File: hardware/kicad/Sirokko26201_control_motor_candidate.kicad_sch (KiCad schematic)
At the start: 35 parts, among them J1 DEVKITC1_J1, J10 TC_K_EXHAUST_T+_T-, J11 TC_K_AIR_T+_T-, J12 ROOM_DS18B20_HARNESS, J13 24V_INPUT_PHOENIX_1756993_WIP, J27 GLOW_OUTPUT_PHOENIX_1756993, J28 CLUTCH_OUTPUT_PHOENIX_1756993, J3 DEVKITC1_J3, K1 DG85BM-5021-76-1024 + DZ85AB-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, K2 DG85BM-5021-76-1024 + DZ85AB-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, Q20 BC847B,215, U10 MAX31856MUD+, U20 SN74LVC1G97DBVR, U9 MAX31856MUD+

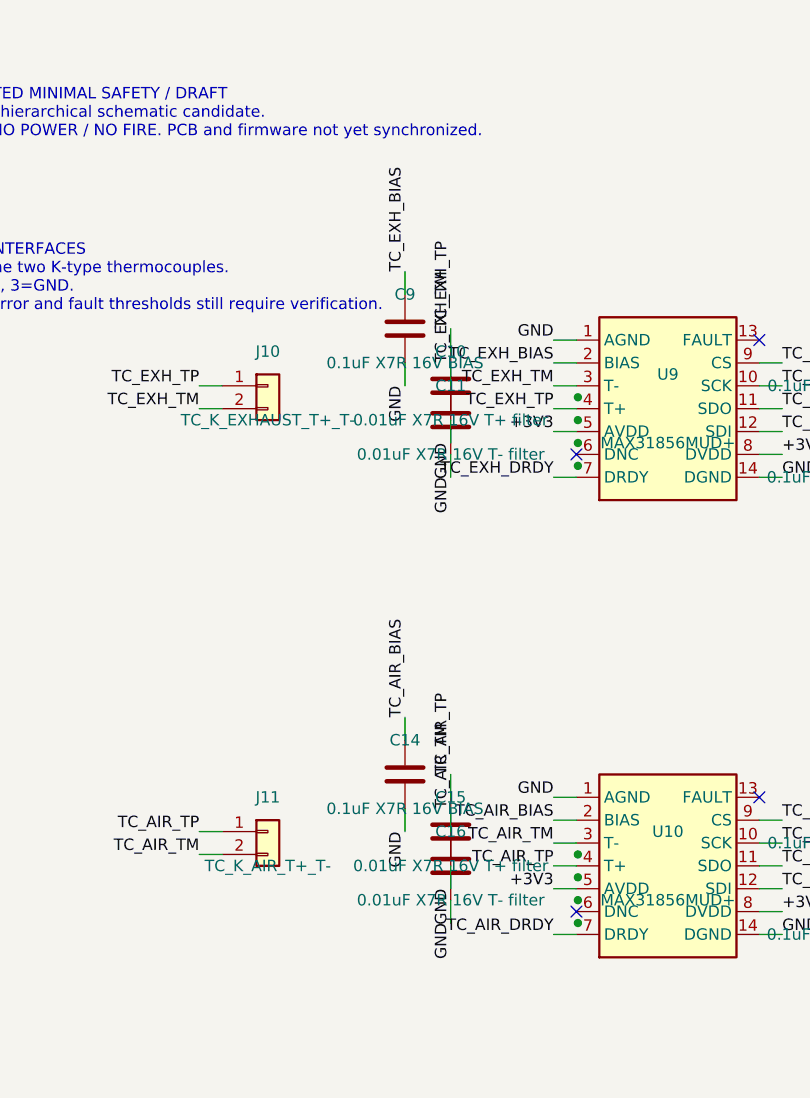
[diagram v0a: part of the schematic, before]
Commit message: Publish thermocouple correction draft package
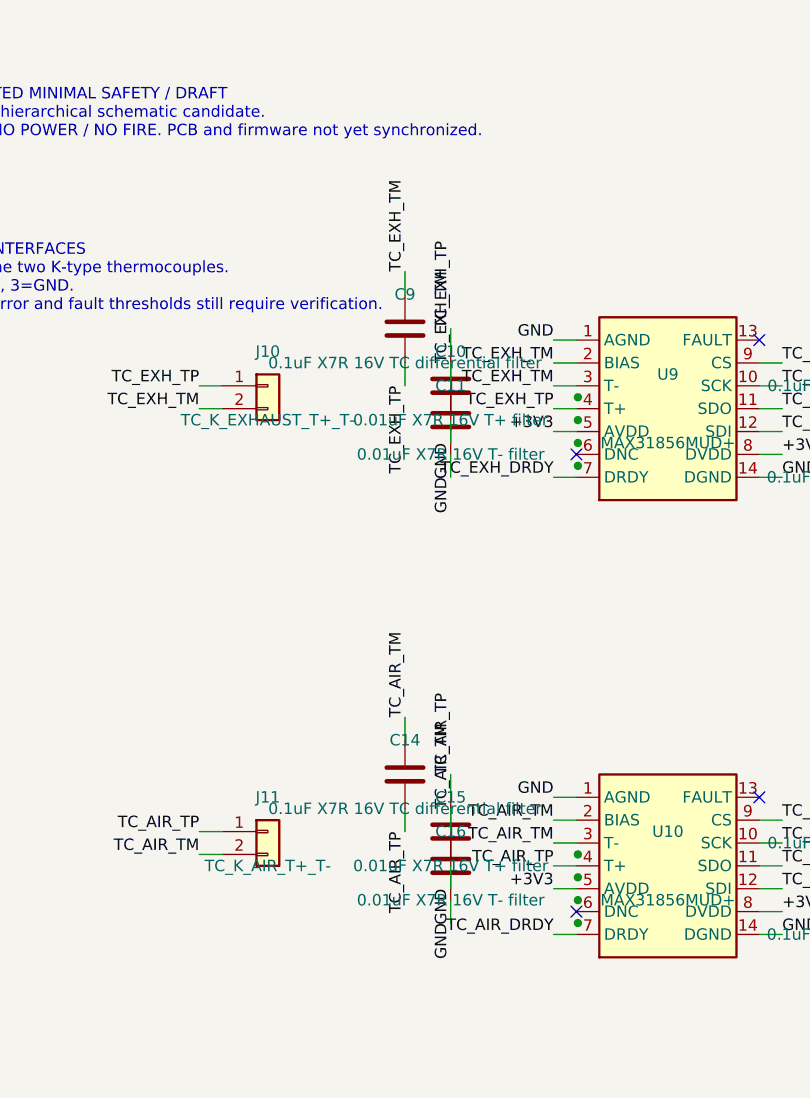
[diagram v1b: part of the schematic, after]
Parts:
- C14, C9: value 0.1uF X7R 16V BIAS -> 0.1uF X7R 16V TC differential filter
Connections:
- net TC_AIR_BIAS is gone; now on net TC_AIR_TM: C14.1, U10.2 (BIAS)
- net TC_EXH_BIAS is gone; now on net TC_EXH_TM: C9.1, U9.2 (BIAS)
- net GND: no longer C14.2, C9.2
- net TC_AIR_TP: now also C14.2
- net TC_EXH_TP: now also C9.2

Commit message: Publish modular MAX31856 schematic WIP
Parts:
- removed C10, C15: 0.01uF X7R 16V T+ filter, Capacitor_SMD:C_0603_1608Metric, symbol Device:C
- removed C11, C16: 0.01uF X7R 16V T- filter, Capacitor_SMD:C_0603_1608Metric, symbol Device:C
- removed C12, C17: 0.1uF X7R 16V AVDD, Sirokko_TFT_Passives:C_Murata_GRM188_1608_Reflow, symbol Device:C
- removed C13, C18: 0.1uF X7R 16V DVDD, Sirokko_TFT_Passives:C_Murata_GRM188_1608_Reflow, symbol Device:C
- removed C14, C9: 0.1uF X7R 16V TC differential filter, Sirokko_TFT_Passives:C_Murata_GRM188_1608_Reflow, symbol Device:C
- removed J10: TC_K_EXHAUST_T+_T-, TerminalBlock_Phoenix:TerminalBlock_Phoenix_MKDS-1,5-2-5.08_1x02_P5.08mm_Horizontal, symbol Sirokko_Interface:Conn_01x02_Sirokko
- removed J11: TC_K_AIR_T+_T-, TerminalBlock_Phoenix:TerminalBlock_Phoenix_MKDS-1,5-2-5.08_1x02_P5.08mm_Horizontal, symbol Sirokko_Interface:Conn_01x02_Sirokko
- removed U10, U9: MAX31856MUD+, Package_SO:TSSOP-14_4.4x5mm_P0.65mm, symbol Sirokko_thermal:MAX31856MUD_PLUS_GRID
- added J30: MAX31856 EXHAUST, Connector_PinSocket_2.54mm:PinSocket_1x09_P2.54mm_Vertical, symbol Connector_Generic:Conn_01x09
- added J31: MAX31856 AIR, Connector_PinSocket_2.54mm:PinSocket_1x09_P2.54mm_Vertical, symbol Connector_Generic:Conn_01x09
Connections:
- net +3V3: now also J30.9 (Pin_9), J31.9 (Pin_9)
- net GND: now also J30.7 (Pin_7), J31.7 (Pin_7)
- net TC_AIR_CS: now also J31.3 (Pin_3)
- net TC_AIR_DRDY: now also J31.1 (Pin_1)
- net TC_EXH_CS: now also J30.3 (Pin_3)
- net TC_EXH_DRDY: now also J30.1 (Pin_1)
- net TC_SCK: now also J30.6 (Pin_6), J31.6 (Pin_6)
- net TC_SDI_MOSI: now also J30.4 (Pin_4), J31.4 (Pin_4)
- net TC_SDO_MISO: now also J30.5 (Pin_5), J31.5 (Pin_5)
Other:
- note added: "RELAY DRIVER DRAFT / NO POWER / NO FLASH / NO FIRE U11 DRV8803: GLOW_CMD to IN1; FUEL_CMD to IN2; IN3/IN4, nENBL and RESET to GND. Exactly K1 glow and K2 clutch; no independent welded-contact cutoff. Driver, relay-coil, transient and thermal qualification remain open."
- note added: "REMOTE CONTROL / MAIN-POWER MONITOR - DRAFT U20 monitors P24 presence; USB power paths remain unqualified. External watchdog/latch and hardware ARM_PULSE logic have been removed. Do not restore obsolete permission circuitry. No physical tests performed."
- note added: "THERMOCOUPLES: J30 EXHAUST / J31 AIR - TYPE K 9-pin MAX31856 modules; Adafruit 3263 geometry. VIN=3V3; 3Vo/FLT=NC; thermocouples at module terminals. J12 DS18B20 unchanged. PCB pending. NO POWER / NO FLASH / NO FIRE."
- note removed: "MINIMUM HARDWARE PERMISSION - DRAFT U1 watchdog; U2 asynchronous-clear latch; U6 three AND gates. U11 is the coil driver. U20 P24 presence monitor retained: USB can keep ESP32 alive during main-power loss. Return of any permission does not itself re-arm the latch; require a fresh ARM_PULSE. The majority of process protections belongs to the ESP32 state machine, not extra logic ICs."
- note removed: "ON-BOARD TEMPERATURE INTERFACES U9/U10 are MAX31856 for the two K-type thermocouples. J12: 1=3V3, 2=DS18B20 DQ, 3=GND. Probe wiring, cold-junction error and fault thresholds still require verification."
- note removed: "RELAY DRIVER DRAFT / NO POWER / NO FIRE U11 DRV8803PWPR: nENBL=HIGH disables all sinks. U2 Q -> SAFETY_OK -> U11 IN3. U2 /Q -> RELAY_DISABLE -> U11 nENBL. GLOW_CMD -> U11 IN1; FUEL_CMD -> U11 IN2; commands remain separate. C21=100nF/100V; C22=330uF/63V. Driver limits, coil release, transient and thermal tests pending. The former U12/U14 gating and C23/C26 bypasses are removed, not silently bypass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"
